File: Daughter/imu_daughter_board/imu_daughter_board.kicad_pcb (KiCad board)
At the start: 2 copper layers, 41.5 x 20 mm, 44 parts, among them IC1 TCAN3413DRBR, J1 Conn_01x04, J2 Conn_ARM_JTAG_SWD_10, Q1 HL2309, SW1 SW_SPST, U1 STM32F103C8Tx, U2 LSM6DSL, U3 TPS5430DDA, X1 SMD3225-4

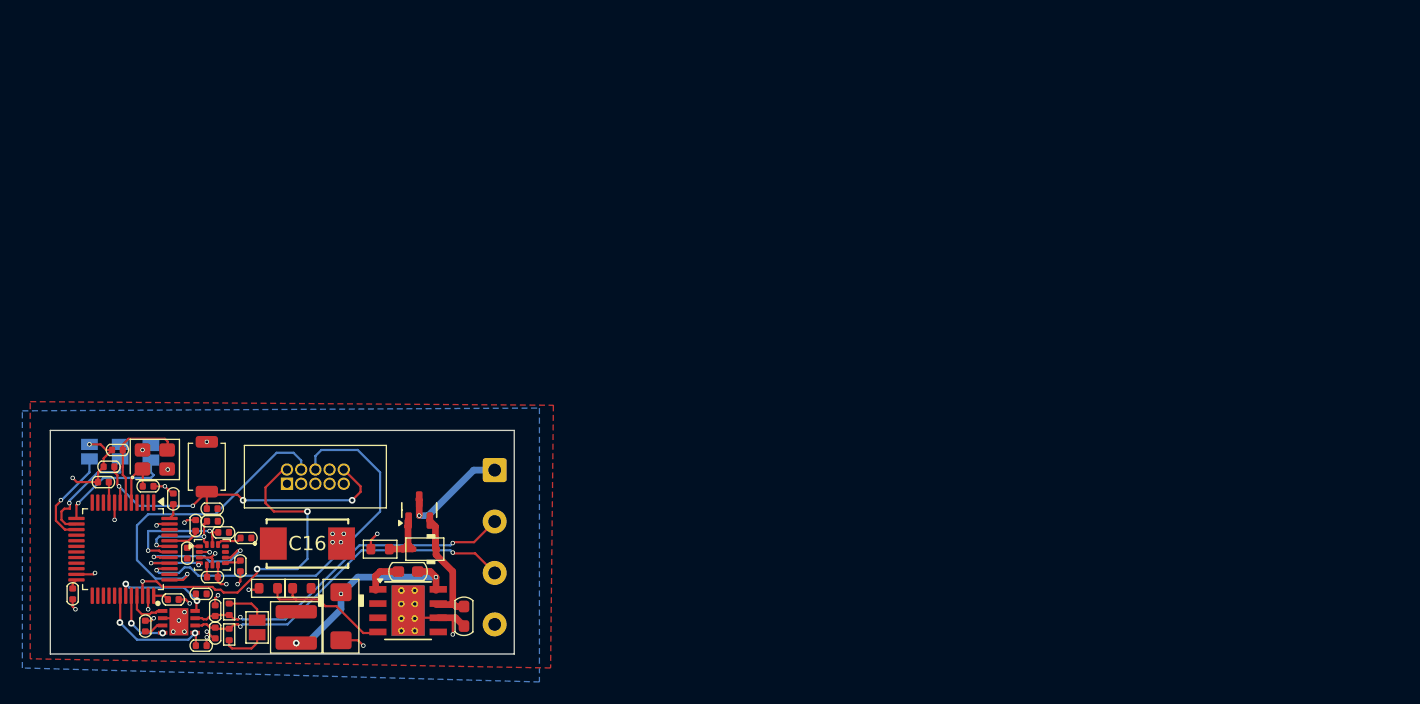
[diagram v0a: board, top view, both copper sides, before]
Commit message: done needs review, all the errors are all related to footprint or pink overlap looks good in 3d
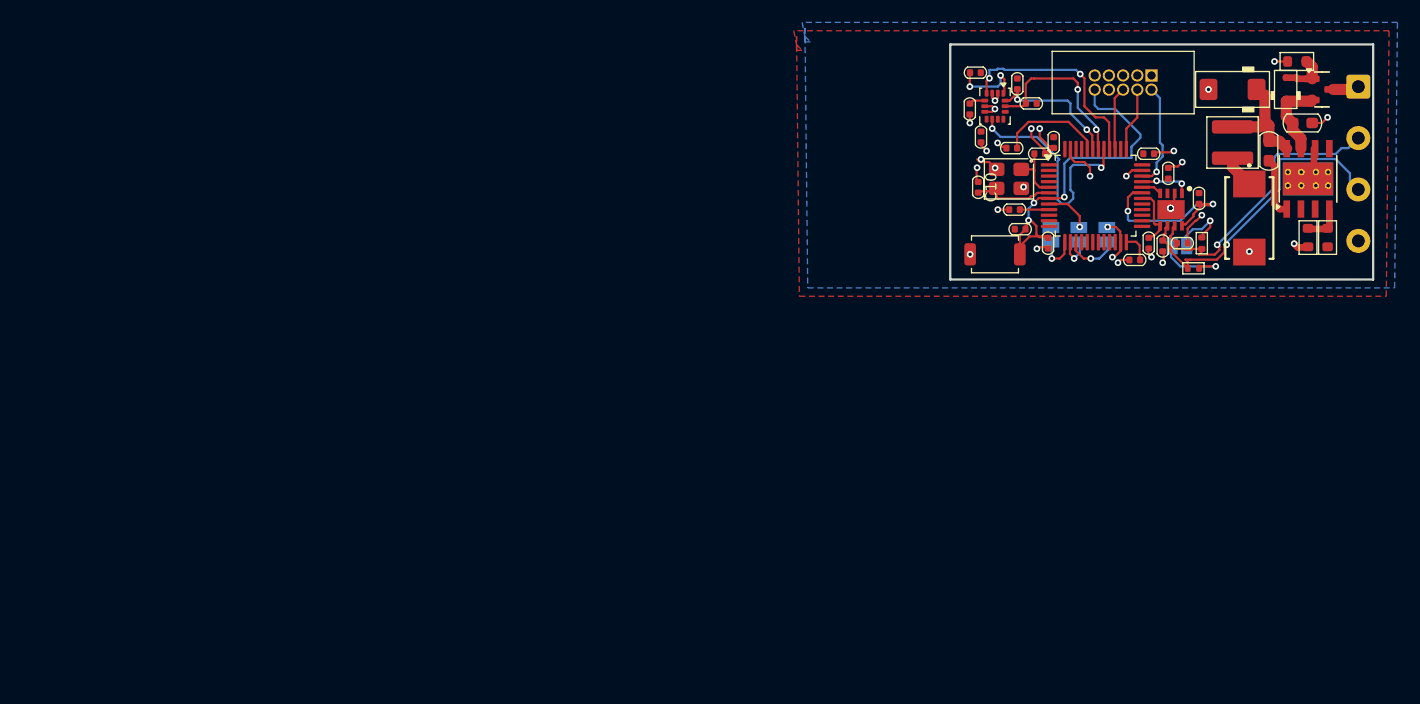
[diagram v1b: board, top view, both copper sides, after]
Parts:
- removed R1: 10k, PCM_Capacitor_SMD_AKL:C_0402_1005Metric
- J1: moved to F.Cu
- JP1: moved to B.Cu
- moved C9 104.0 mm to (228.2, 65.2), turned to 0 degrees
- moved C5 100.1 mm to (230.0, 67.0)
- moved R12 98.1 mm to (242.5, 72.8), turned to -90 degrees
- moved R11 97.0 mm to (244.2, 72.8), turned to 90 degrees
- moved IC1 96.1 mm to (230.2, 70.2), turned to -90 degrees
- moved R7 96.0 mm to (232.8, 69.2), turned to -90 degrees
- moved L1 94.3 mm to (235.8, 64.2), turned to -90 degrees
- moved JP2 93.0 mm to (224.5, 72.5)
- moved R5 93.0 mm to (233.0, 73.2)
- moved R13 92.9 mm to (241.5, 57.0)
- moved D1 92.6 mm to (235.8, 59.5), turned to 180 degrees
- moved U1 92.6 mm to (223.5, 69.0), turned to 0 degrees
- moved C4 92.5 mm to (231.2, 73.2), turned to 180 degrees
- moved R6 92.3 mm to (232.2, 75.5), turned to 180 degrees
- moved R8 92.1 mm to (228.2, 73.2), turned to -90 degrees
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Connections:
- U2 pad 12: Net-(U2-CS) -> 3.3V
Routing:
- net /SWO: track 35.8 -> 5.50 mm, vias 1 -> 0
- net /SWCLK: track 28.8 -> 5.72 mm, vias 1 -> 0
- net /SWDIO: track 30.2 -> 9.44 mm, vias 3 -> 1
- net /INT1: track 5.98 -> 18.8 mm
- net /INT2: track 11.4 -> 21.2 mm
- net Net-(D1-K): track 18.8 -> 9.25 mm, vias 3 -> 0
- net Net-(U3-VSENSE): track 12.0 -> 3.54 mm
- net VIN: track 9.92 -> 2.35 mm, vias 1 -> 0
- net Net-(JP3-B): track 10.6 -> 3.35 mm
- net /STB: track 9.64 -> 16.7 mm
- net Net-(JP4-B): track 10.7 -> 3.97 mm
- net Net-(U1-BOOT0): track 2.87 -> 9.48 mm
- net /SHDNVIO: track 11.3 -> 5.47 mm, vias 2 -> 0
- net Net-(U2-SDO/SA0): track 1.14 -> 6.84 mm, vias 0 -> 2
- net /CANP: track 31.0 -> 26.4 mm, vias 2 -> 1
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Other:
- board size 41.5 x 20 mm -> 37.8 x 21 mm
- board text removed: "Main Sheet"
